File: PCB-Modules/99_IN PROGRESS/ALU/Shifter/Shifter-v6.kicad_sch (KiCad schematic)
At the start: 33 parts, among them J1 Conn_01x08, J2 Conn_01x08, J3 Conn_01x07, U1 74LS08, U2 74LS194, U3 74LS194, U4 74LS86, U5 74LS245

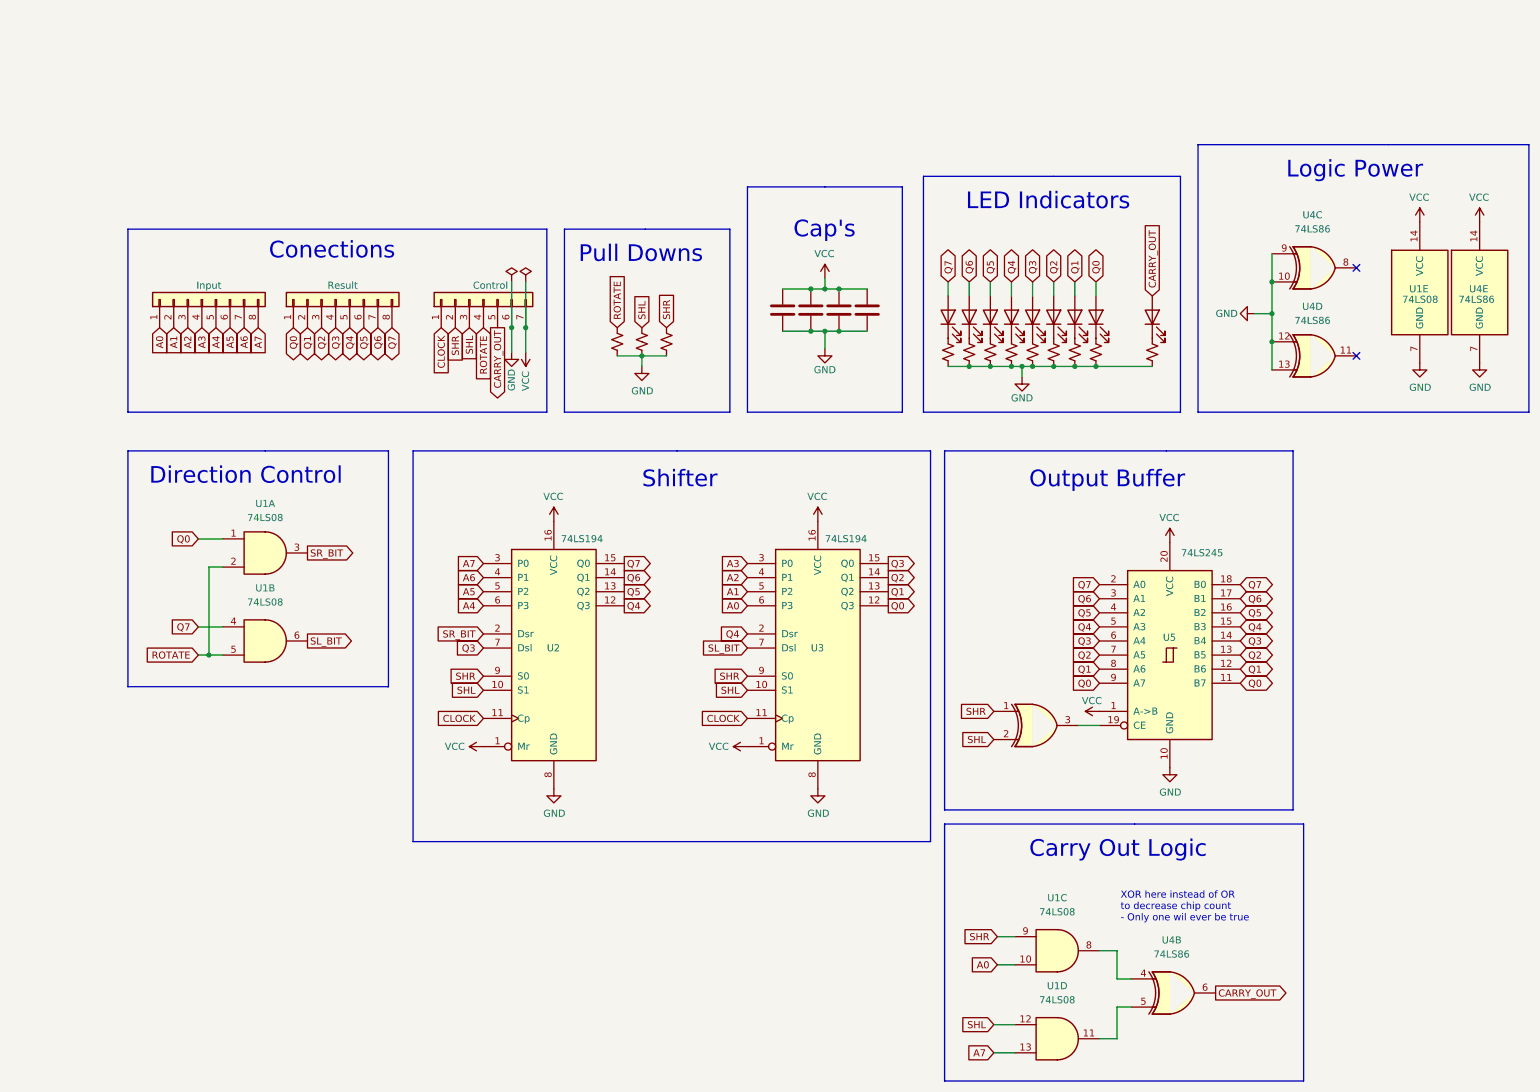
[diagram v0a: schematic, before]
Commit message: Documentation and Cleanup
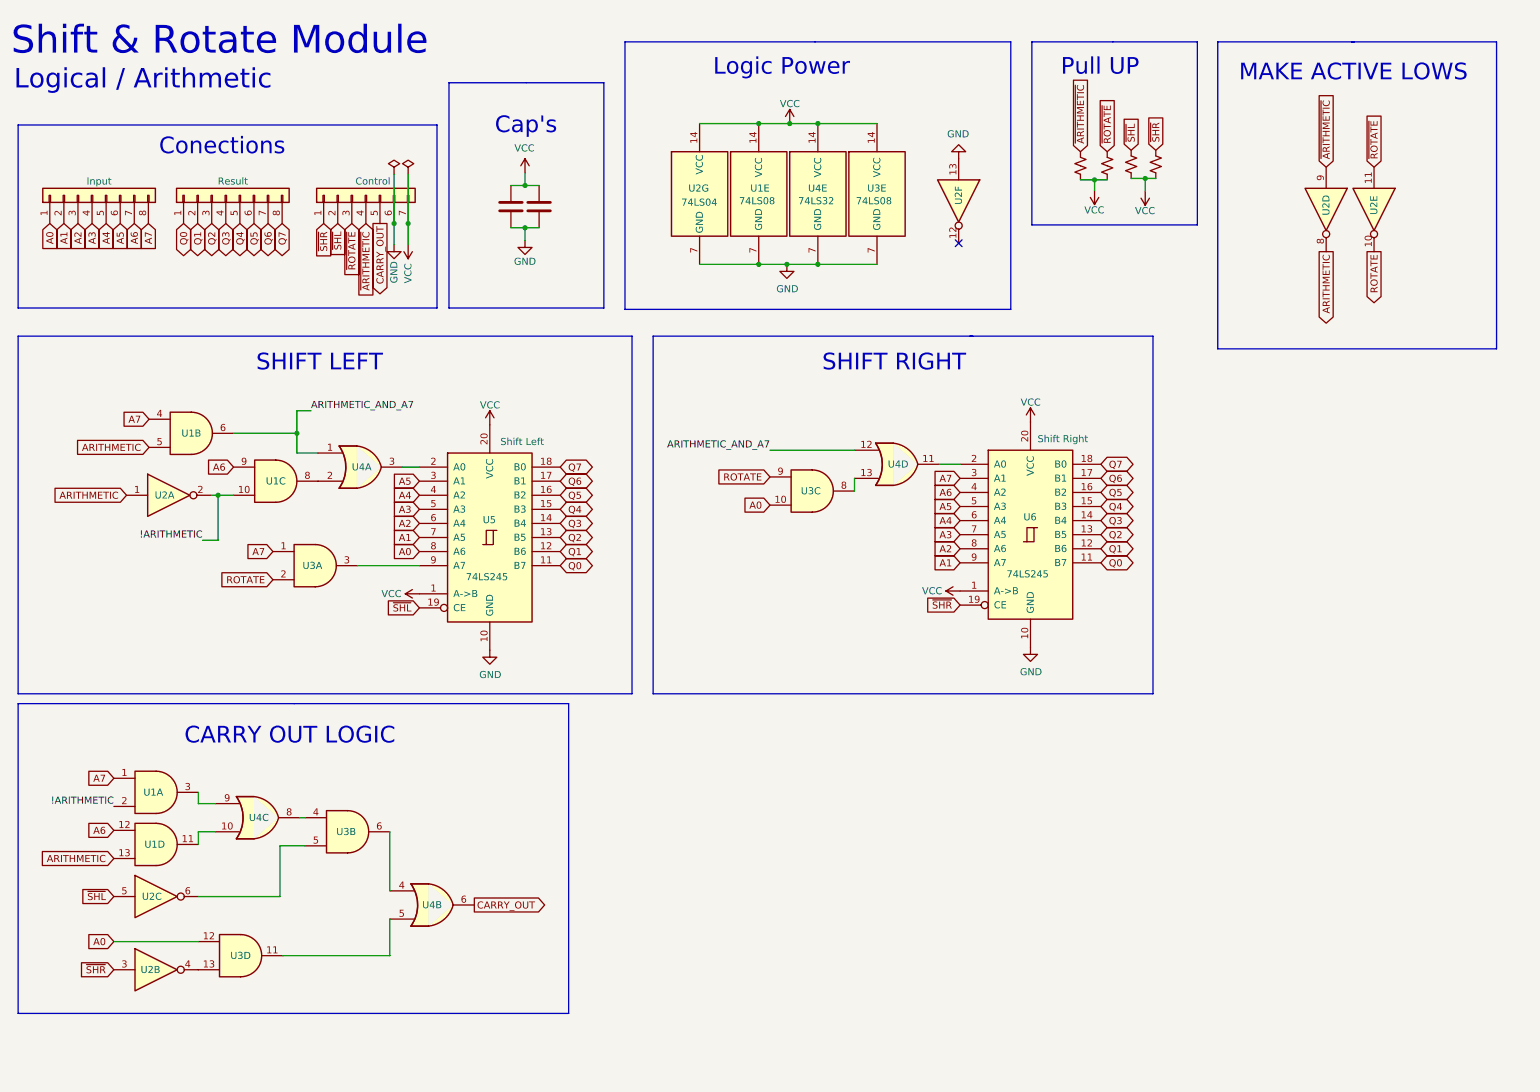
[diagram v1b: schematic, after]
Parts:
- removed C? (x2): C, Capacitor_SMD:C_0805_2012Metric, symbol Device:C
- removed D1, D2, D3, D4, D5, D6, D7, D8, D?: LED, LED_SMD:LED_0805_2012Metric, symbol Device:LED
- removed R1, R2, R3, R4, R5, R6, R7, R8, R?: R_Small_US, Resistor_SMD:R_0805_2012Metric, symbol Device:R_Small_US
- removed U2, U3: 74LS194, Package_SO:SOIC-16_4.55x10.3mm_P1.27mm, symbol 74xx:74LS194
- removed U4: 74LS86, Package_SO:TSSOP-14_4.4x5mm_P0.65mm, symbol 74xx:74LS86
- added R13: R_Small_US, Resistor_SMD:R_0805_2012Metric, symbol Device:R_Small_US
- added U2: 74LS04, Package_SO:TSSOP-14_4.4x5mm_P0.65mm, symbol 74xx:74LS04
- added U3: 74LS08, Package_SO:TSSOP-14_4.4x5mm_P0.65mm, symbol 74xx:74LS08
- added U4: 74LS32, Package_SO:TSSOP-14_4.4x5mm_P0.65mm, symbol 74xx:74LS32
- added U6: 74LS245, Package_SO:TSSOP-20_4.4x5mm_P0.5mm, symbol 74xx:74LS245
- U5: Func (none) -> Shift Left
- gave numbers to parts that had none: 5
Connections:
- net A0: now also U5.8 (A6), U3.10, U3.12; no longer U1.10
- net A1: now also U5.7 (A5), U6.9 (A7)
- net A2: now also U5.6 (A4), U6.8 (A6)
- net A3: now also U5.5 (A3), U6.7 (A5)
- net A4: now also U5.4 (A2), U6.6 (A4)
- net A5: now also U5.3 (A1), U6.5 (A3)
- net A6: now also U1.12, U1.9, U6.4 (A2)
- net A7: now also U1.1, U1.4, U3.1, U6.3 (A1); no longer U1.13
- net CARRY_OUT: now also U4.6
- net GND: now also U2.13, U2.7 (GND), U3.7 (GND), U4.7 (GND), U6.10 (GND); no longer R10.2, R11.2, R12.2
- net Q0: now also U6.11 (B7); no longer U1.1, U5.9 (A7)
- net Q1: now also U6.12 (B6); no longer U5.8 (A6)
- net Q2: now also U6.13 (B5); no longer U5.7 (A5)
- net Q3: now also U6.14 (B4); no longer U5.6 (A4)
- net Q4: now also U6.15 (B3); no longer U5.5 (A3)
- net Q5: now also U6.16 (B2); no longer U5.4 (A2)
- net Q6: now also U6.17 (B1); no longer U5.3 (A1)
- net Q7: now also U6.18 (B0); no longer U1.4, U5.2 (A0)
- net ROTATE: now also U2.10, U3.2, U3.9; no longer J3.4 (Pin_4), R10.1, U1.2, U1.5
- net VCC: now also R10.2, R11.2, R12.2, R13.2, U2.14 (VCC), U3.14 (VCC), U4.14 (VCC), U6.1 (A->B), U6.20 (VCC)
- net ~{SHL}: now reaches U5.19 (CE)
- net ~{SHL}: now also J3.2 (Pin_2), R11.1, U2.5
- net at U1.8: now also U4.2
- net at U1.11: now also U4.10
- net CLOCK renamed ~{SHR}
- net ~{SHR}: now also R12.1, U2.3, U6.19 (CE)
- removed net SHL: J3.3 (Pin_3), R11.1, U1.12
- removed net SHR: J3.2 (Pin_2), R12.1, U1.9
- net SL_BIT renamed ARITHMETIC_AND_A7
- net ARITHMETIC_AND_A7: now also U4.1, U4.12
- net SR_BIT: no longer names the net of U1.3
- net SR_BIT: now also U4.9
- new net: U3.11, U4.5
- new net: U2.4, U3.13
- new net: U3.4, U4.8
- new net: U4.11, U6.2 (A0)
- new net: U3.8, U4.13
- new net: U4.3, U5.2 (A0)
- new net: U2.6, U3.5
- new net: U3.6, U4.4
- new net: U3.3, U5.9 (A7)
- new net !ARITHMETIC: U1.10, U1.2, U2.2
- new net ARITHMETIC: U1.13, U1.5, U2.1, U2.8
- new net ~{ARITHMETIC}: J3.4 (Pin_4), R13.1, U2.9
- new net ~{ROTATE}: J3.3 (Pin_3), R10.1, U2.11
- no-connect marks 2 -> 1
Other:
- note added: "CARRY OUT LOGIC"
- note added: "Logical / Arithmetic"
- note added: "MAKE ACTIVE LOWS"
- note added: "Pull UP"
- note added: "SHIFT LEFT"
- note added: "SHIFT RIGHT"
- note added: "Shift & Rotate Module"
- note removed: "Carry Out Logic"
- note removed: "Direction Control"
- note removed: "LED Indicators"
- note removed: "Output Buffer"
- note removed: "Pull Downs"
- note removed: "Shifter"
- note removed: "XOR here instead of OR to decrease chip count - Only one wil ever be true"
- company: (none) -> theWickedWebDev/8-bit-computer
- title: (none) -> Arithmetic & Logical Shifter Module
